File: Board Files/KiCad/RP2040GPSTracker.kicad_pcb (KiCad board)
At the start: 2 copper layers, 99.6 x 53 mm, 123 parts, among them J1 BOOTSEL, J10 GNSS, J11 GPIO9-15, J2 RESET, J3 DEBUG, J4 BT(LE), J5 GSM, J6 USBC_CHARGE, J7 USBC_PROG, J8 2822541-1, J9 BATTERY, U1 W25Q128JVS, U10 LM66200DRLR, U2 SIM868, U3 RP2040, U4 SN74LVC1G66DRYR, U5 LM66200DRLR, U6 MP2624GL, U7 NCP1117LPST33T3G, U8 SAFFB1G56KB0F5F, Y1 Crystal

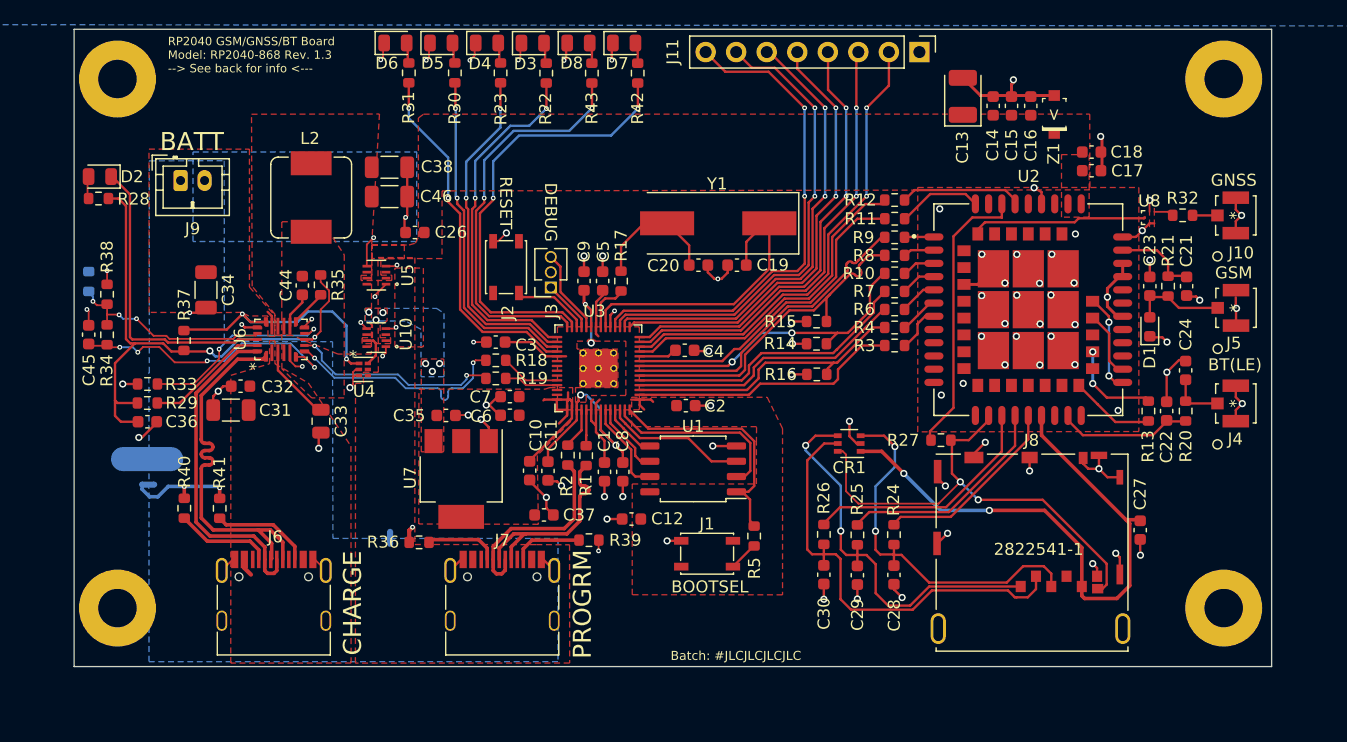
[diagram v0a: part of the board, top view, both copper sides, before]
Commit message: Rev 2.0
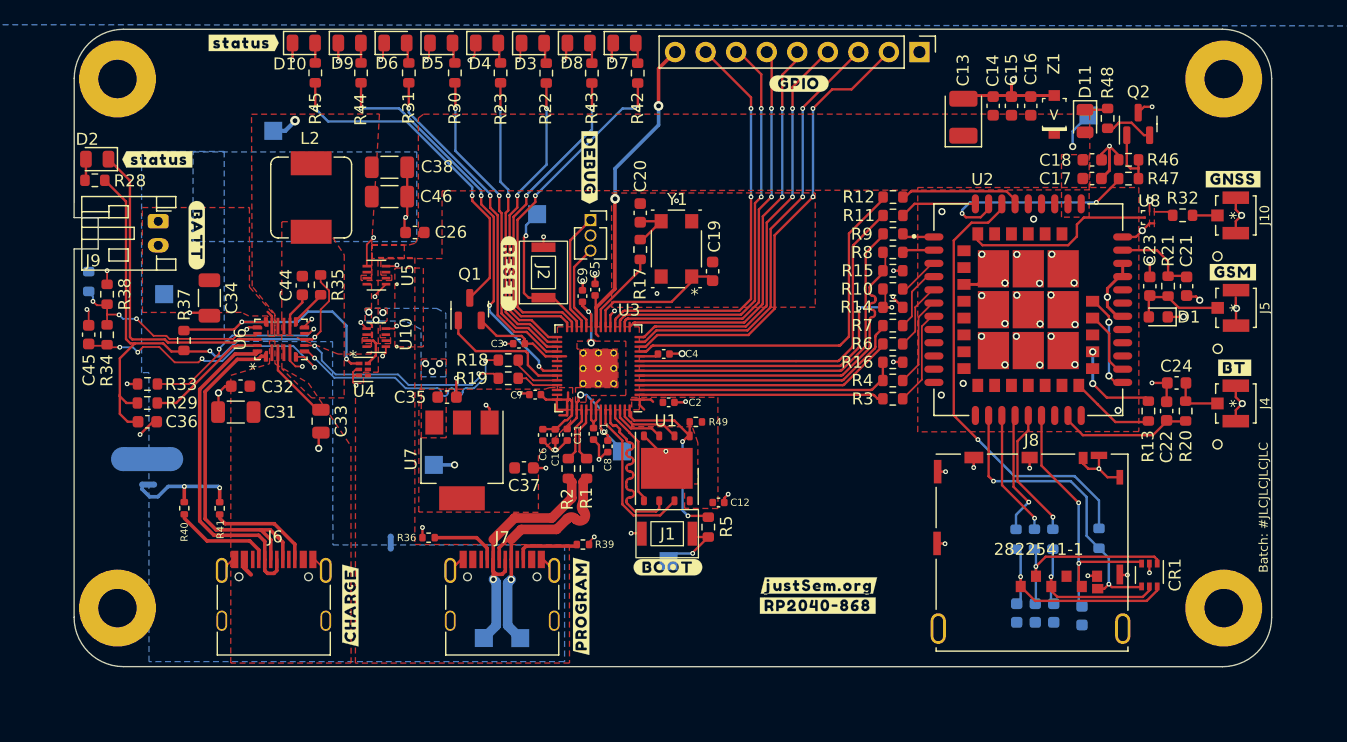
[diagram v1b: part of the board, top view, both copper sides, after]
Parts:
- added ?: , RP2040-868Graphics:charge-fs, F.Cu at (94.4, 55.5)
- added ?: , RP2040-868Graphics:bt-re, F.Cu at (166.2, 32.0)
- added ?: , RP2040-868Graphics:gnss-re, F.Cu at (165.2, 16.3)
- added ?: , RP2040-868Graphics:program-fs, F.Cu at (113.6, 56.2)
- added ?: , RP2040-868Graphics:batt-ca, F.Cu at (81.6, 18.1)
- added ?: , RP2040-868Graphics:debug-ha, F.Cu at (114.3, 12.0)
- added ?: , RP2040-868Graphics:r2_0-ca, B.Cu at (136.1, 53.4)
- added ?: , RP2040-868Graphics:date-cc-ha, B.Cu at (141.9, 55.1)
- added ?: , RP2040-868Graphics:rev-cc-ha, B.Cu at (141.9, 53.4)
- added ?: , RP2040-868Graphics:9-ca, B.Cu at (139.2, 9.81)
- added ?: , RP2040-868Graphics:14-ca, B.Cu at (126.4, 10.5)
- added ?: , RP2040-868Graphics:status-lc-ha-left, F.Cu at (75.4, 14.7)
- added ?: , RP2040-868Graphics:12-ca, B.Cu at (131.5, 10.5)
- added ?: , RP2040-868Graphics:wikiref-re, B.Cu at (126.7, 28.2)
- added ?: , RP2040-868Graphics:15-ca, B.Cu at (123.9, 10.4)
- added ?: , RP2040-868Graphics:3v3-lc-ca, B.Cu at (121.4, 11.8)
- added ?: , RP2040-868Graphics:gnd-ca, B.Cu at (141.7, 12.1)
- added ?: , RP2040-868Graphics:13-ca, B.Cu at (129.0, 10.5)
- added ?: , RP2040-868Graphics:11-ca, B.Cu at (134.1, 10.3)
- added ?: , RP2040-868Graphics:10-ca, B.Cu at (136.6, 10.5)
- added ?: , RP2040-868Graphics:status-lc-ha, F.Cu at (82.2, 4.99)
- added ?: , RP2040-868Graphics:gsm-re, F.Cu at (165.5, 24.1)
- added ?: , RP2040-868Graphics:gpio-ca, F.Cu at (129.2, 8.38)
- added ?: , RP2040-868Graphics:boot-ca, F.Cu at (117.9, 48.6)
- added ?: , RP2040-868Graphics:reset-ca, F.Cu at (107.6, 21.1)
- added ?: , RP2040-868Graphics:rp2040-868-re, F.Cu at (128.1, 51.8)
- added ?: , RP2040-868Graphics:jsorg-fs, F.Cu at (128.2, 50.1)
- added D10: BLUE, LED_SMD:LED_0805_2012Metric, F.Cu at (90.5, 5.00)
- added D11: BLUE, LED_SMD:LED_0805_2012Metric, F.Cu at (155.5, 11.5)
- added D9: BLUE, LED_SMD:LED_0805_2012Metric, F.Cu at (94.3, 5.00)
- added Q1: Si2319CDS, Package_TO_SOT_SMD:SOT-23, F.Cu at (104.3, 27.1)
- added Q2: Si2319CDS, Package_TO_SOT_SMD:SOT-23, F.Cu at (159.9, 11.7)
- added R44: 20, Resistor_SMD:R_0603_1608Metric, F.Cu at (95.3, 7.49)
- added R45: 100, Resistor_SMD:R_0603_1608Metric, F.Cu at (91.5, 7.49)
- added R46: 47k, Resistor_SMD:R_0603_1608Metric, F.Cu at (159.1, 14.7)
- added R47: 4.7k, Resistor_SMD:R_0603_1608Metric, F.Cu at (159.1, 16.3)
- added R48: 56, Resistor_SMD:R_0603_1608Metric, F.Cu at (157.3, 11.3)
- added R49: DNF, Resistor_SMD:R_0402_1005Metric, F.Cu at (123.1, 36.5)
- added REF**: Symbol_CC-Attribution_SilkscreenTop_Small, Symbol:Symbol_CC-Attribution_SilkscreenTop_Small, B.Cu at (127.0, 39.6)
- added REF**: Symbol_CreativeCommons_SilkscreenTop_Type2_Small, Symbol:Symbol_CreativeCommons_SilkscreenTop_Type2_Small, B.Cu at (142.0, 39.6)
- added REF**: Symbol_CC-Noncommercial_SilkscreenTop_Small, Symbol:Symbol_CC-Noncommercial_SilkscreenTop_Small, B.Cu at (97.0, 39.6)
- added REF**: Symbol_CC-ShareAlike_SilkscreenTop_Small, Symbol:Symbol_CC-ShareAlike_SilkscreenTop_Small, B.Cu at (112.0, 39.6)
- added TP1: TestPoint, TestPoint:TestPoint_Pad_1.5x1.5mm, B.Cu at (105.5, 54.5)
- added TP2: TestPoint, TestPoint:TestPoint_Pad_1.5x1.5mm, B.Cu at (108.5, 54.5)
- added TP3: TestPoint, TestPoint:TestPoint_Pad_1.5x1.5mm, B.Cu at (117.0, 39.0)
- added TP4: TestPoint, TestPoint:TestPoint_Pad_1.5x1.5mm, B.Cu at (101.3, 40.1)
- added TP5: TestPoint, TestPoint:TestPoint_Pad_1.5x1.5mm, B.Cu at (155.8, 11.0)
- added TP6: TestPoint, TestPoint:TestPoint_Pad_1.5x1.5mm, B.Cu at (109.9, 19.2)
- added TP7: TestPoint, TestPoint:TestPoint_Pad_1.5x1.5mm, B.Cu at (120.8, 48.1)
- added TP8: TestPoint, TestPoint:TestPoint_Pad_1.5x1.5mm, B.Cu at (88.0, 12.3)
- added TP9: TestPoint, TestPoint:TestPoint_Pad_1.5x1.5mm, B.Cu at (78.9, 25.9)
- C1, C10, C11, C12, C2, C3, C4, C5, C6, C7, C8, C9: footprint Capacitor_SMD:C_0603_1608Metric -> Capacitor_SMD:C_0402_1005Metric
- C27, C28, C29, C30, R24, R25, R26, R27: moved to B.Cu
- D3, D7, D8: value LED -> RED
- D4, D5, D6: value LED -> BLUE
- J1, J2: footprint Button_Switch_SMD:TS-1145A-C-A -> Button_Switch_SMD:SW_SPST_ALPS_SKRKAEE020
- J11: footprint Connector_PinHeader_2.54mm:PinHeader_1x08_P2.54mm_Vertical -> Connector_PinHeader_2.54mm:PinHeader_1x09_P2.54mm_Vertical
- J9: footprint Connector_JST:JST_PH_B2B-PH-K_1x02_P2.00mm_Vertical -> Connector_JST:JST_PH_S2B-PH-K_1x02_P2.00mm_Horizontal
- R22, R42, R43: value 330 -> 56
- R23, R30, R31: value 330 -> 20
- R28: value 1k -> 100/0.2
- R36, R39, R40, R41: value 5.6k -> 5.1k; footprint Resistor_SMD:R_0603_1608Metric -> Resistor_SMD:R_0402_1005Metric
- U1: footprint Package_SO:SOIC-8_5.23x5.23mm_P1.27mm -> Package_SON:WSON-8-1EP_6x5mm_P1.27mm_EP3.4x4.3mm
- Y1: footprint Crystal:Crystal_SMD_HC49-SD -> ABRACON:ABMM2-12.000MHZ-E2-T
- moved CR1 27.3 mm to (160.8, 49.2), turned to -90 degrees
- moved C30 17.9 mm to (151.3, 52.4)
- moved R26 17.5 mm to (151.3, 46.3)
- moved R27 15.5 mm to (156.6, 46.2), turned to -90 degrees
- moved C28 13.7 mm to (152.9, 52.4)
- moved C29 13.6 mm to (149.8, 52.4)
- moved R24 13.2 mm to (152.8, 46.3)
- moved R25 13.2 mm to (149.7, 46.3)
- moved C27 8.61 mm to (155.2, 52.6)
- moved R15 7.62 mm to (139.5, 23.9), turned to 180 degrees
- moved C12 7.37 mm to (125.0, 43.2), turned to 0 degrees
- moved R14 7.03 mm to (139.5, 27.0), turned to 180 degrees
- moved C20 6.51 mm to (118.5, 19.1), turned to 90 degrees
- moved J3 6.50 mm to (114.3, 19.7), turned to 0 degrees
- moved R16 6.40 mm to (139.5, 31.6), turned to 180 degrees
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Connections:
- net Net-(J2-Pad1) renamed /PI_RESET
- net Net-(R1-Pad2) renamed /PI_D+
- net Net-(R2-Pad2) renamed /PI_D-
- net Net-(R22-Pad2) renamed /LED_3
- net Net-(R23-Pad2) renamed /LED_4
- net Net-(R30-Pad2) renamed /LED_5
- net Net-(R31-Pad2) renamed /LED_6
- net Net-(R5-Pad1) renamed /SPI_SS
- net Net-(U1-Pad2) renamed /SPI_IO1
- net Net-(U1-Pad3) renamed /SPI_IO2
- net Net-(U1-Pad5) renamed /SPI_IO0
- net Net-(U1-Pad6) renamed /SPI_CLK
- net Net-(U1-Pad7) renamed /SPI_IO3
- net Net-(U3-Pad27) renamed /LED_1
- net Net-(U3-Pad28) renamed /LED_2
- C20 pad 1: Net-(C20-Pad1) -> Net-(Y1-Pad3)
- CR1 pad 1: /SIM_C_VDD -> Net-(C30-Pad2)
- CR1 pad 3: Net-(C28-Pad2) -> /SIM_C_VDD
- CR1 pad 4: Net-(C29-Pad2) -> /SIM_C_DET
- CR1 pad 5: Net-(C30-Pad2) -> Net-(C28-Pad2)
- CR1 pad 6: /SIM_C_DET -> Net-(C29-Pad2)
- R17 pad 2: Net-(C20-Pad1) -> Net-(Y1-Pad3)
- U2 pad 41: unconnected-(U2-Pad41) -> /SIM_NETLIGHT
- U3 pad 36: unconnected-(U3-Pad36) -> /LED_7
- U3 pad 37: unconnected-(U3-Pad37) -> /LED_PWR
- Y1 pad 2: Net-(C20-Pad1) -> GND
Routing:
- net /LED_7: track 0.00 -> 33.5 mm, vias 0 -> 4
- net Net-(Q1-Pad3): track 0.00 -> 28.4 mm, vias 0 -> 2
- net /SIM_C_VDD: track 48.6 -> 24.6 mm
- net +3V3: track 37.4 -> 58.6 mm, vias 0 -> 3
- net Net-(C30-Pad2): track 37.4 -> 16.3 mm, vias 0 -> 1
- net /SIM_NETLIGHT: track 0.00 -> 17.5 mm, vias 0 -> 2
- net GND: track 137.1 -> 120.2 mm, vias 92 -> 90
- net Net-(C28-Pad2): track 31.7 -> 14.8 mm, vias 2 -> 1
- net Net-(C29-Pad2): track 33.4 -> 18.2 mm, vias 2 -> 1
- net /SIM_C_DET: track 40.7 -> 25.9 mm
- net /SIM_VDD_EXT: track 23.6 -> 37.4 mm, vias 0 -> 1
- net Net-(U3-Pad20): track 24.7 -> 11.9 mm
- net /LED_PWR: track 0.00 -> 11.3 mm
- net Net-(C20-Pad1): track 10.9 -> 0.00 mm
- net /SPI_IO1: track 15.6 -> 5.38 mm
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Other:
- outline, holes or cut-outs redrawn
- board text added: "+1.1V"
- board text added: "+3.3V"
- board text added: "+4V"
- board text added: "+5V"
- board text added: "24"
- board text added: "25"
- board text added: "26-03-2022"
- board text added: "800mA max!"
- board text added: "BOOT"
- board text added: "D+ D-"
- board text added: "Get started at"
- board text added: "LED D10"
- board text added: "LED D9"
- board text added: "PGND"
- board text added: "RUN"
- board text added: "STATUS"
- board text removed: "10"
- board text removed: "11"
- board text removed: "12"
- board text removed: "13"
- board text removed: "14"
- board text removed: "15"
- board text removed: "9"
- board text removed: "BATT"
- board text removed: "BOOTSEL"
- board text removed: "Board Rev.: 1.3 18-03-2022"
- board text removed: "CHARGE"
- board text removed: "DEBUG"
- board text removed: "GND"
- board text removed: "GPIO#:"
- board text removed: "Get started at wiki.justsem.org/rp2040-868"
- board text removed: "PROGRM"
- board text removed: "RESET"
- board text removed: "RP2040 GSM/GNSS/BT Board Model: RP2040-868 Rev. 1.3 --> See back for info <---"
